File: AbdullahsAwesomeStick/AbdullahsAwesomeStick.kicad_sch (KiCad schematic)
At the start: 22 parts, among them J2 AVR-ISP-6, J5 Conn_01x04_Socket, P1 Conn_01x03_Pin, P2 Conn_01x03_Pin, P3 Conn_01x03_Pin, P4 Conn_01x03_Pin, SW1 SW_Push_Open_Dual, U3 ATmega328P-A, Y2 Resonator

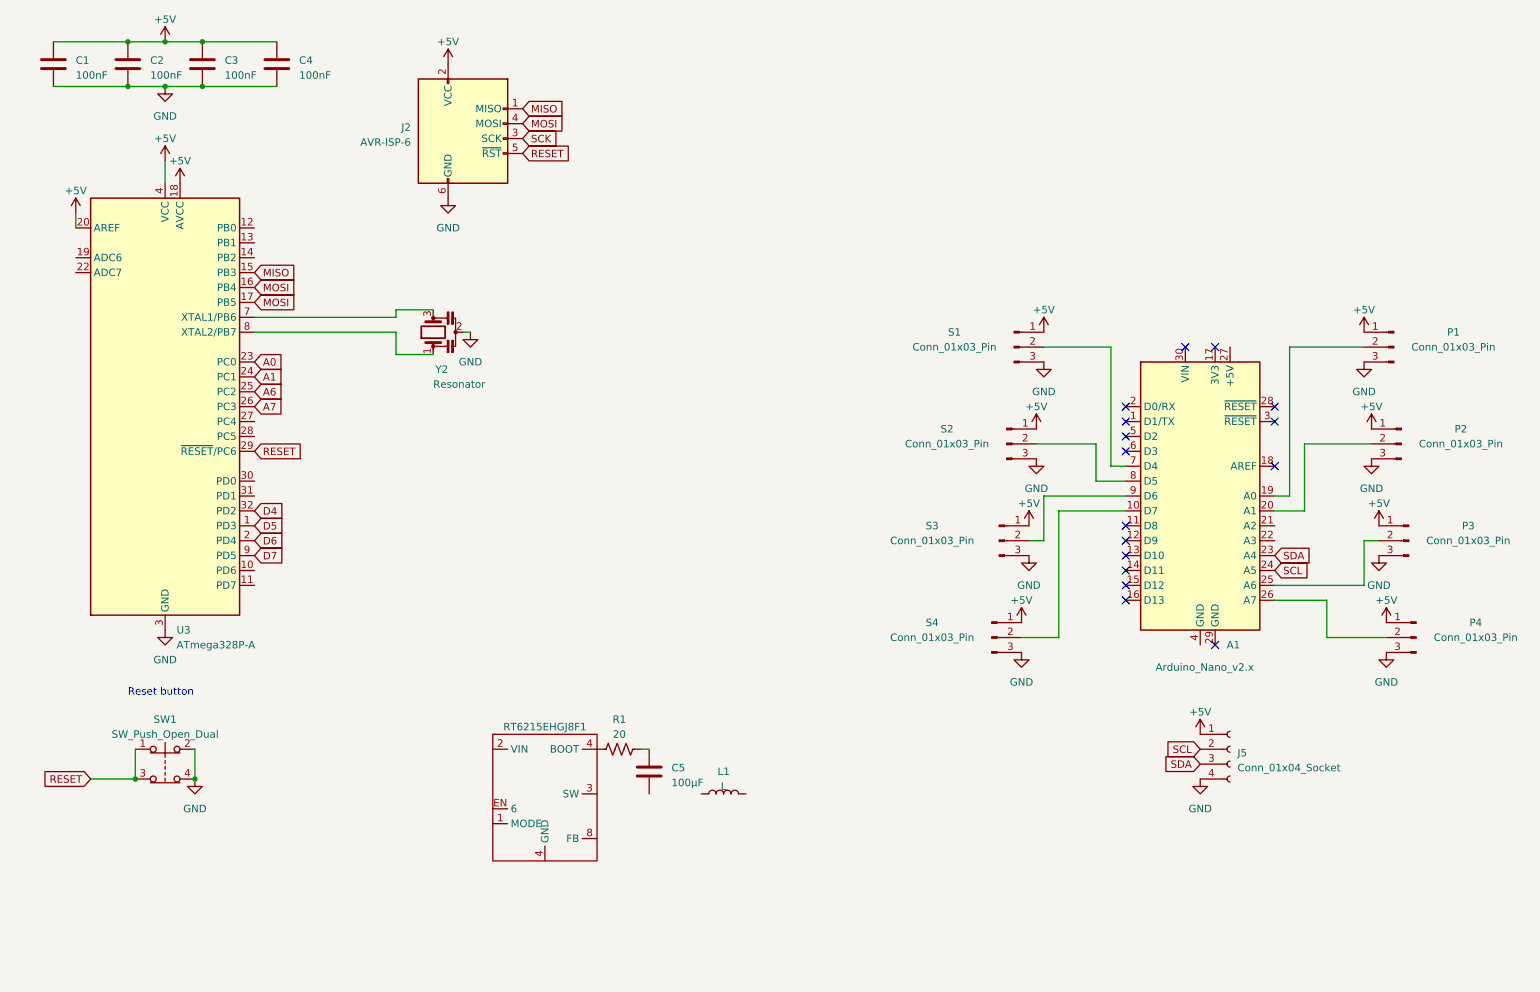
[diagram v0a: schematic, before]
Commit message: Add files via upload
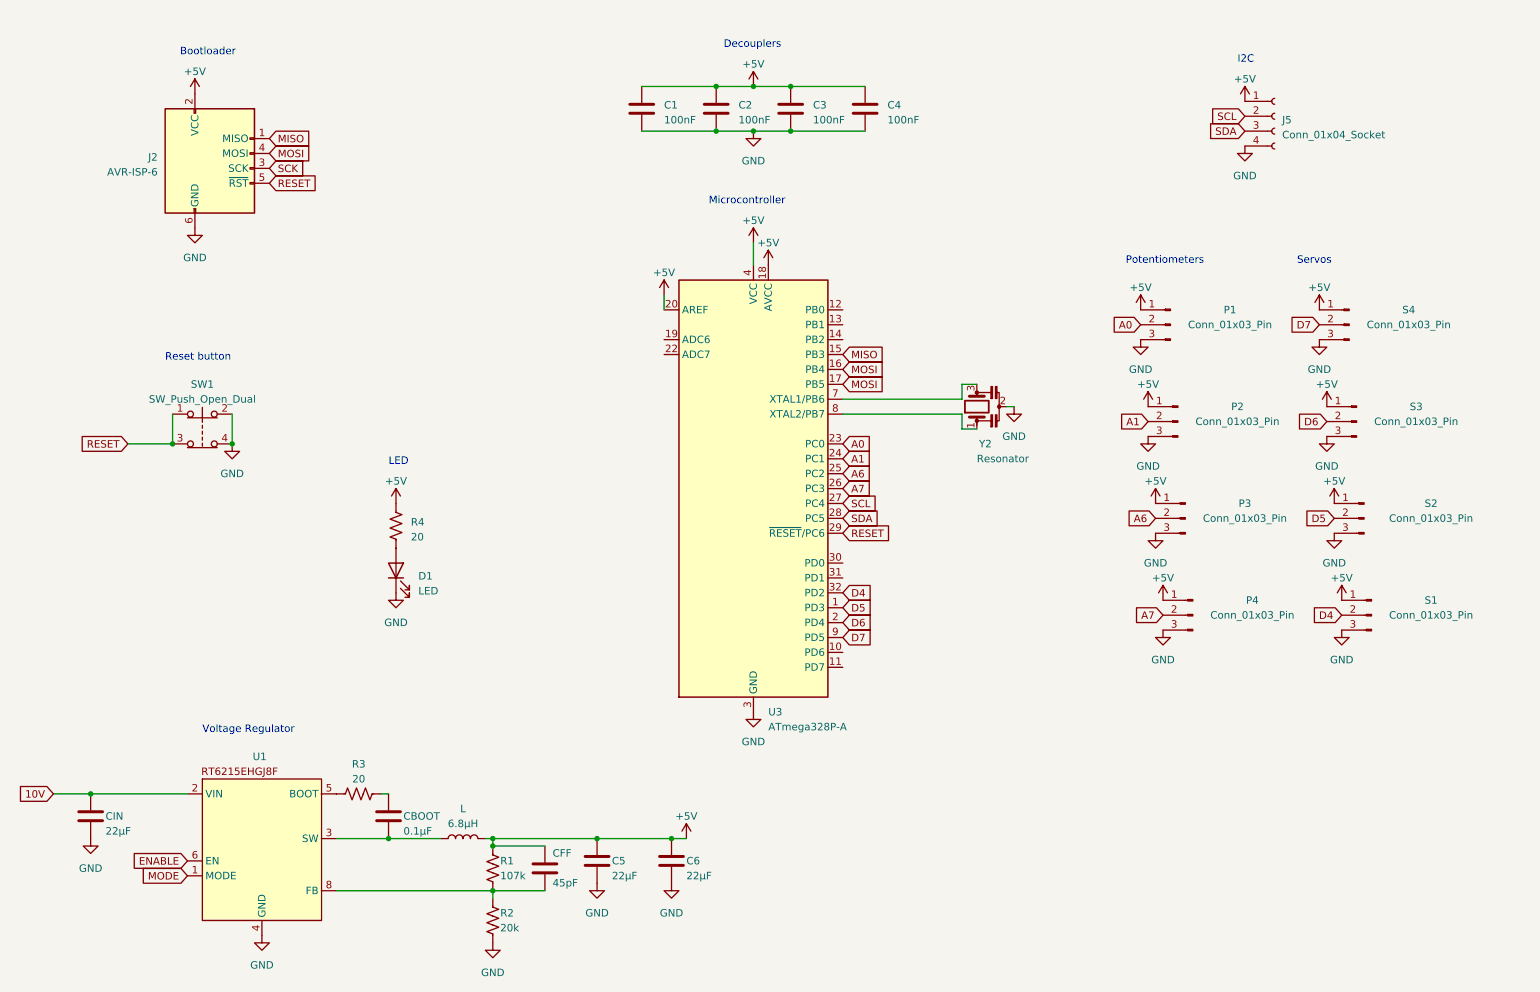
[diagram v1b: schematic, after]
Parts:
- removed A1: Arduino_Nano_v2.x, Module:Arduino_Nano, symbol MCU_Module:Arduino_Nano_v2.x
- removed RT6215EHGJ8F1: ~, symbol Regulators:RT6215EHGJ8F
- added C5, C6, CIN: 22µF, symbol Device:C
- added CFF: 45pF, symbol Device:C
- added D1: LED, symbol Device:LED
- added R1: 107k, symbol Device:R_US
- added R2: 20k, symbol Device:R_US
- added R4: 20, symbol Device:R_US
- added U1: ~, symbol Regulators:RT6215EHGJ8F
- CBOOT: renamed from C5; value 100µF -> 0.1µF
- L: renamed from L1; value L -> 6.8µH
- renumbered R1 to R3
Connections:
- net +5V: now also L.2, C5.1, C6.1, CFF.1, R1.2, R4.2
- net A0: now also P1.2 (Pin_2)
- net A1: now also P2.2 (Pin_2)
- net A6: now also P3.2 (Pin_2)
- net A7: now also P4.2 (Pin_2)
- net D4: now also S1.2 (Pin_2)
- net D5: now also S2.2 (Pin_2)
- net D6: now also S3.2 (Pin_2)
- net D7: now also S4.2 (Pin_2)
- net GND: now also C5.2, C6.2, CIN.2, D1.1 (K), R2.1, U1.4 (GND)
- net SCL: now also U3.27 (PC4)
- net SDA: now also U3.28 (PC5)
- net at CBOOT.2: now also L.1, U1.3 (SW)
- net at R3.1: now also U1.5 (BOOT)
- new net: CFF.2, R1.1, R2.2, U1.8 (FB)
- new net: D1.2 (A), R4.1
- new net 10V: CIN.1, U1.2 (VIN)
- new net ENABLE: U1.6 (EN)
- new net MODE: U1.1 (MODE)
- no-connect marks 16 -> 0
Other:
- note added: "Bootloader"
- note added: "Decouplers"
- note added: "I2C"
- note added: "LED"
- note added: "Microcontroller"
- note added: "Potentiometers"
- note added: "Servos"
- note added: "Voltage Regulator"
- moved on the sheet: C1, C2, C3, C4, CBOOT, J2, J5, L, R3, SW1, U3, Y2
